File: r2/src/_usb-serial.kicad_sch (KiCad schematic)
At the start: 10 parts, among them U12 CP2102N-Axx-xQFN24

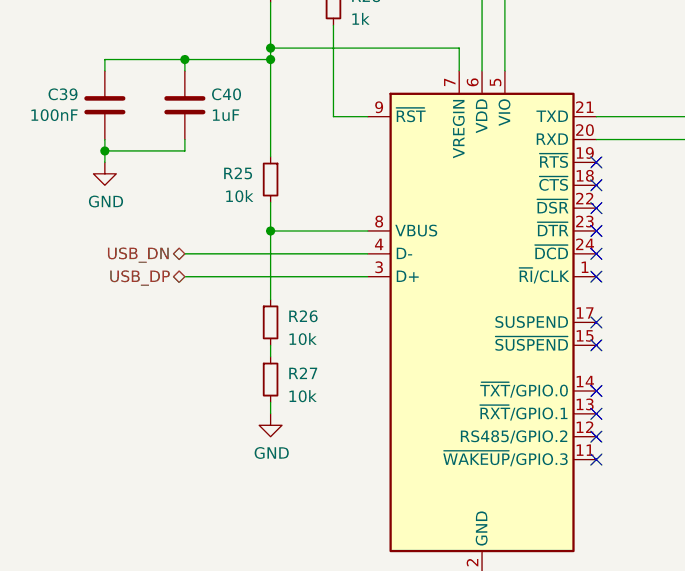
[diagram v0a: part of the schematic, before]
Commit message: Most footprints assigned
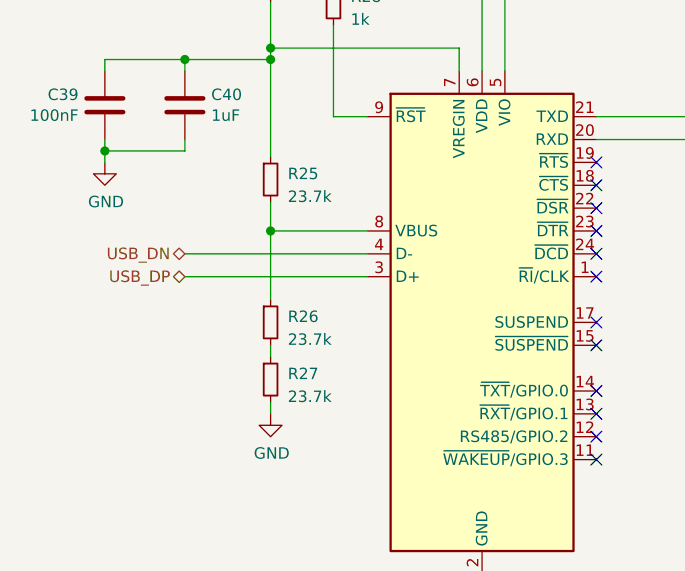
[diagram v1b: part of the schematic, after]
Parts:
- C32, C33, C39: footprint Capacitor_SMD:C_0402_1005Metric -> Capacitor_SMD:C_0603_1608Metric
- R25, R26, R27: value 10k -> 23.7k; footprint (none) -> Resistor_SMD:R_0603_1608Metric
- R28: footprint (none) -> Resistor_SMD:R_0603_1608Metric
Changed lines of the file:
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@@
     (pin "1")
   )
-  (symbol (lib_id "Device:R_Small") (at 119.38 93.98 0) (mirror y) (unit 1)
+  (symbol (lib_id "Device:R_Small") (at 119.38 93.98 0) (unit 1)
     (in_bom yes) (on_board yes)
-    (property "Reference" "R25" (id 0) (at 117.475 93.345 0)
+    (property "Reference" "R25" (id 0) (at 121.285 93.345 0)
       (effects (font (size 1.27 1.27)) (justify left))
     )
-    (property "Value" "10k" (id 1) (at 117.475 95.885 0)
+    (property "Value" "23.7k" (id 1) (at 121.285 95.885 0)
       (effects (font (size 1.27 1.27)) (justify left))
     )
-    (property "Footprint" "" (id 2) (at 119.38 93.98 0)
+    (property "Footprint" "Resistor_SMD:R_0603_1608Metric" (id 2) (at 119.38 93.98 0)
       (effects (font (size 1.27 1.27)) hide)
     )
@@
       (effects (font (size 1.27 1.27)) (justify left))
     )
-    (property "Value" "10k" (id 1) (at 121.285 111.76 0)
+    (property "Value" "23.7k" (id 1) (at 121.285 111.76 0)
       (effects (font (size 1.27 1.27)) (justify left))
     )
-    (property "Footprint" "" (id 2) (at 119.38 109.855 0)
+    (property "Footprint" "Resistor_SMD:R_0603_1608Metric" (id 2) (at 119.38 109.855 0)
       (effects (font (size 1.27 1.27)) hide)
     )
@@
       (effects (font (size 1.27 1.27)) (justify left))
     )
-    (property "Value" "10k" (id 1) (at 121.285 118.11 0)
+    (property "Value" "23.7k" (id 1) (at 121.285 118.11 0)
       (effects (font (size 1.27 1.27)) (justify left))
     )
-    (property "Footprint" "" (id 2) (at 119.38 116.205 0)
+    (property "Footprint" "Resistor_SMD:R_0603_1608Metric" (id 2) (at 119.38 116.205 0)
       (effects (font (size 1.27 1.27)) hide)
     )
@@
       (effects (font (size 1.27 1.27)) (justify left))
     )
-    (property "Footprint" "" (id 2) (at 126.365 74.295 0)
+    (property "Footprint" "Resistor_SMD:R_0603_1608Metric" (id 2) (at 126.365 74.295 0)
       (effects (font (size 1.27 1.27)) hide)
     )
@@
       (effects (font (size 1.27 1.27)) (justify left))
     )
-    (property "Footprint" "Capacitor_SMD:C_0402_1005Metric" (id 2) (at 99.9998 89.535 0)
+    (property "Footprint" "Capacitor_SMD:C_0603_1608Metric" (id 2) (at 99.9998 89.535 0)
       (effects (font (size 1.27 1.27)) hide)
     )
@@
       (effects (font (size 1.27 1.27)) (justify left))
     )
-    (property "Footprint" "Capacitor_SMD:C_0402_1005Metric" (id 2) (at 155.2702 65.405 0)
+    (property "Footprint" "Capacitor_SMD:C_0603_1608Metric" (id 2) (at 155.2702 65.405 0)
       (effects (font (size 1.27 1.27)) hide)
     )
@@
       (effects (font (size 1.27 1.27)) (justify left))
     )
-    (property "Footprint" "Capacitor_SMD:C_0402_1005Metric" (id 2) (at 174.9298 83.185 0)
+    (property "Footprint" "Capacitor_SMD:C_0603_1608Metric" (id 2) (at 174.9298 83.185 0)
       (effects (font (size 1.27 1.27)) hide)
     )
